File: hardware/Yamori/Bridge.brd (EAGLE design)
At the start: 50.5 x 55.9 mm, 10 parts, among them J1 CONN_20X2, U3 SN74LS244N

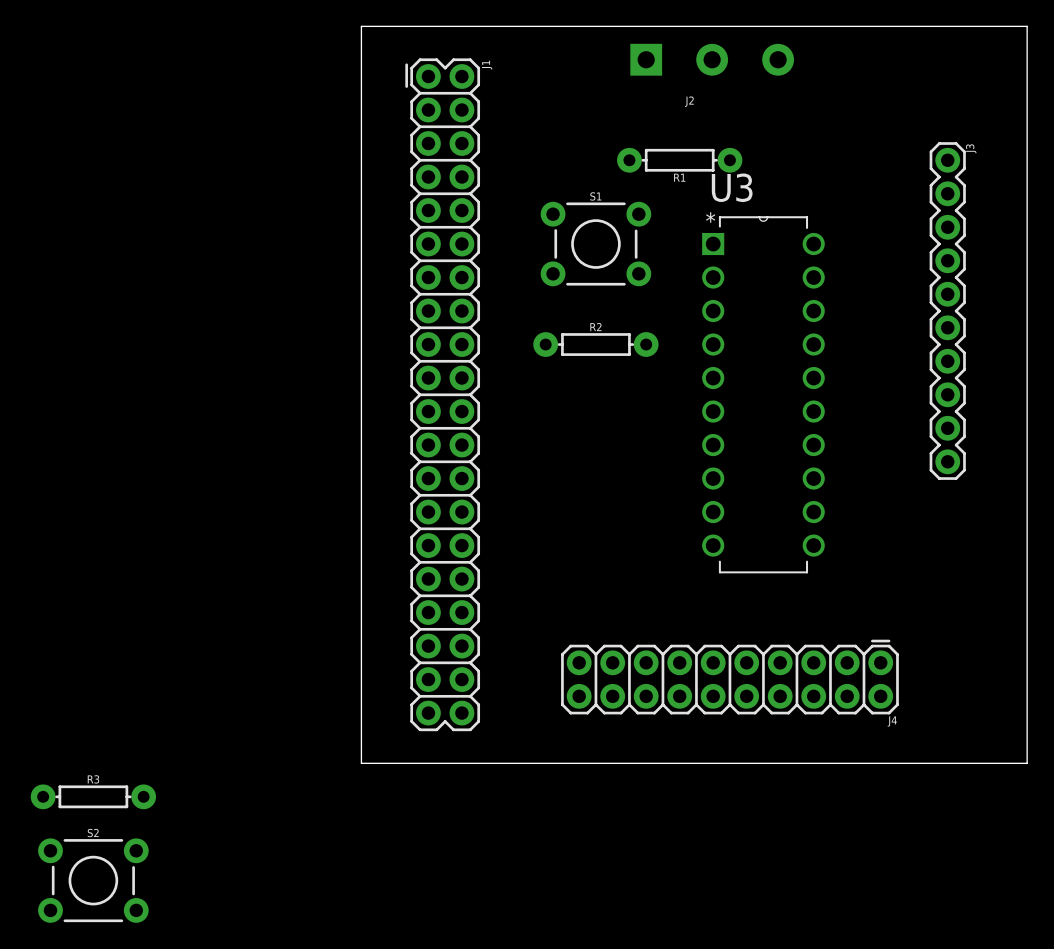
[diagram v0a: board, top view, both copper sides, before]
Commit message: Wiring in progress
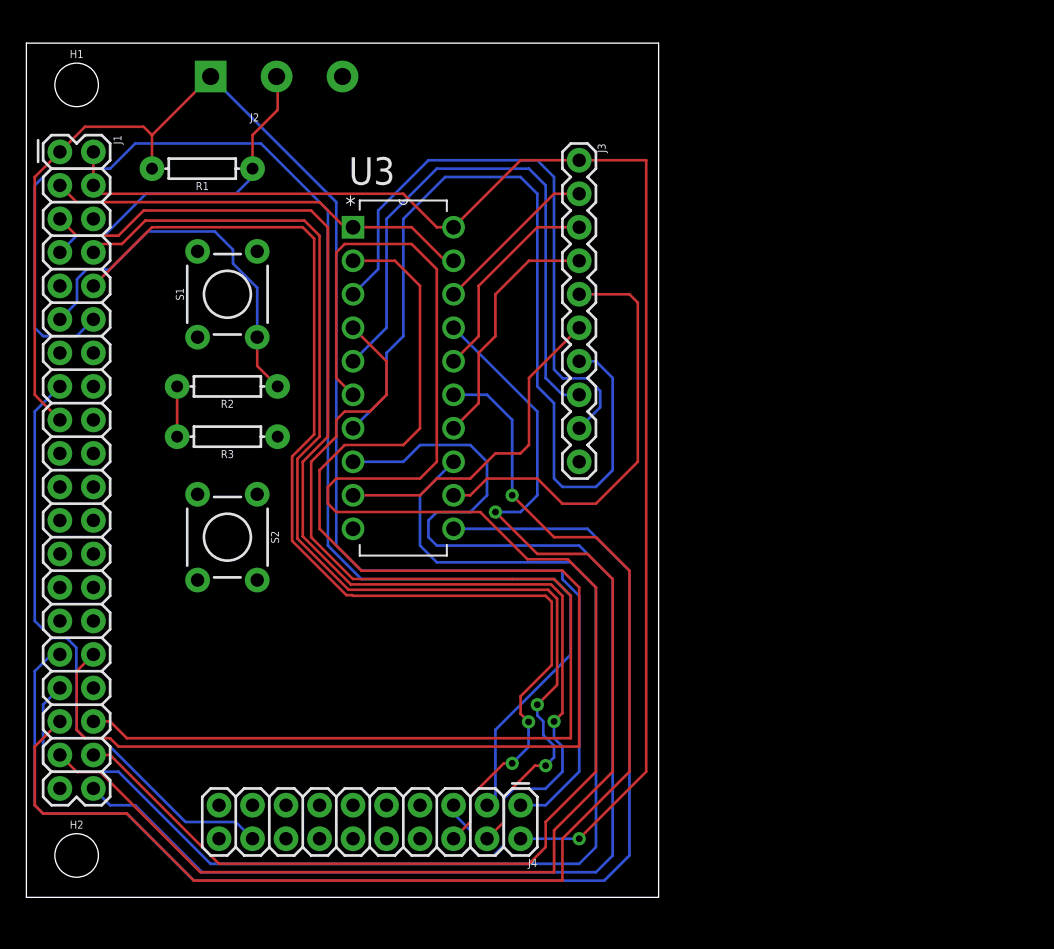
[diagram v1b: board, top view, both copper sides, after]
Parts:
- added H1, H2: STAND-OFF, SparkFun-Hardware:STAND-OFF
- moved R1 36.2 mm to (13.3, 55.2)
- moved J2 33.0 mm to (14.0, 62.2)
- moved J4 29.4 mm to (37.5, 6.99)
- moved R3 29.1 mm to (15.2, 34.9), turned to 180 degrees
- moved J1 28.5 mm to (2.54, 56.5)
- moved S1 28.2 mm to (15.2, 45.7), turned to 90 degrees
- moved R2 28.1 mm to (15.2, 38.7), turned to 180 degrees
- moved S2 27.9 mm to (15.2, 27.3), turned to 270 degrees
- moved J3 27.9 mm to (41.9, 55.9)
- moved U3 27.3 mm to (32.4, 27.9)
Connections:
- net BCM22: now also J4.18
- net BCM24: no longer J4.18
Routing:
- net 1A3: track 0.00 -> 127.4 mm
- net 3.3V: track 0.00 -> 121.3 mm
- net 1A1: track 0.00 -> 108.5 mm
- net 5V: track 0.00 -> 105.9 mm, vias 0 -> 1
- net BCM18: track 0.00 -> 105.6 mm
- net 1A4: track 0.00 -> 99.0 mm
- net BCM3: track 0.00 -> 97.5 mm, vias 0 -> 1
- net 2A3: track 0.00 -> 97.3 mm, vias 0 -> 1
- net 2A1: track 0.00 -> 97.1 mm
- net 2A4: track 0.00 -> 95.2 mm, vias 0 -> 1
- net 2A2: track 0.00 -> 93.6 mm
- net 1A2: track 0.00 -> 89.5 mm
- net BCM15: track 0.00 -> 86.1 mm, vias 0 -> 2
- net BCM14: track 0.00 -> 85.8 mm, vias 0 -> 2
- net 2Y2: track 0.00 -> 66.9 mm
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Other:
- board size 50.5 x 55.9 mm -> 47.9 x 64.8 mm
